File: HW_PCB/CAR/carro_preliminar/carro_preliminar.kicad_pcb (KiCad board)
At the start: 2 copper layers, 33 parts, among them IC1 TB6612FNG, J1 V_Battery, J2 STLINK, J3 Motores, J5 UART, J6 Servo_Motor, J7 NRF24_Con, SW1 SW_DPST_x2, U1 STM32F103C8Tx, U2 AMS1117-3.3, U3 AMS1117-3.3, Y1 8MHz

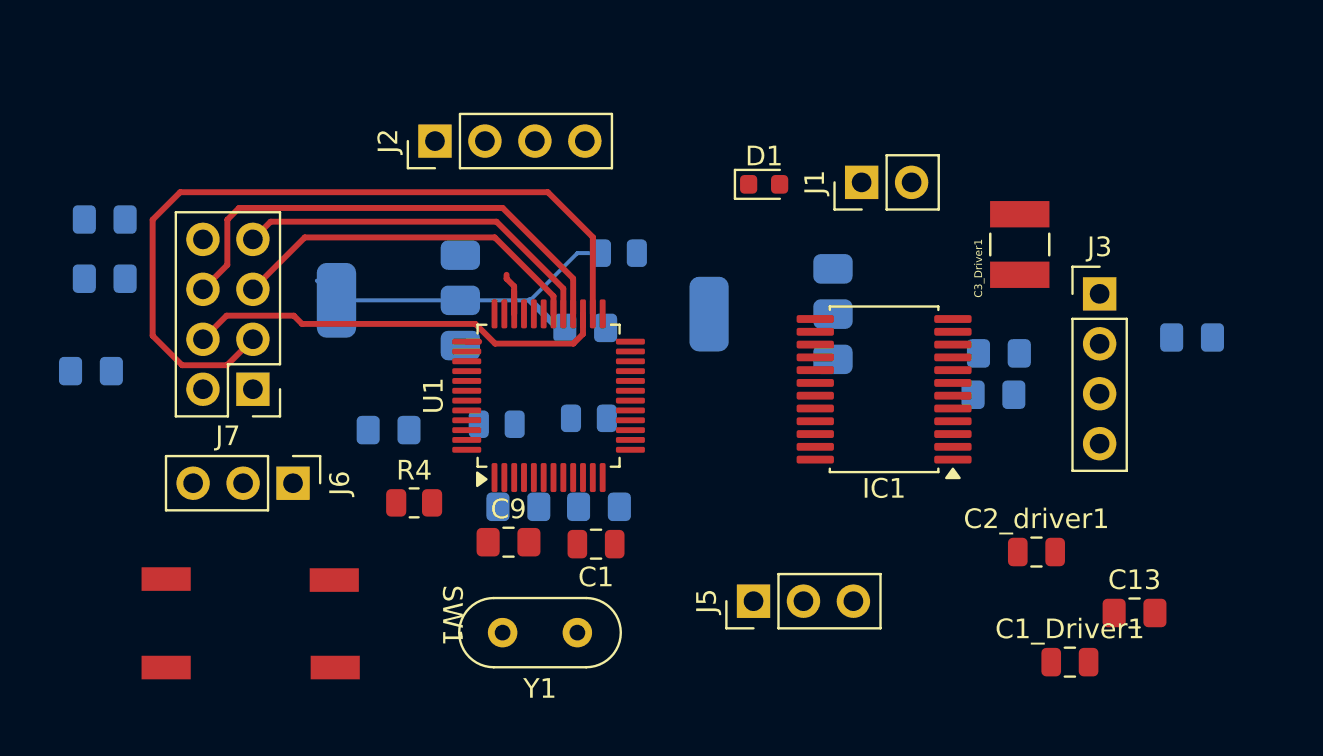
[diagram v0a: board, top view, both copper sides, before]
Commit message: Carrito 26-02-26
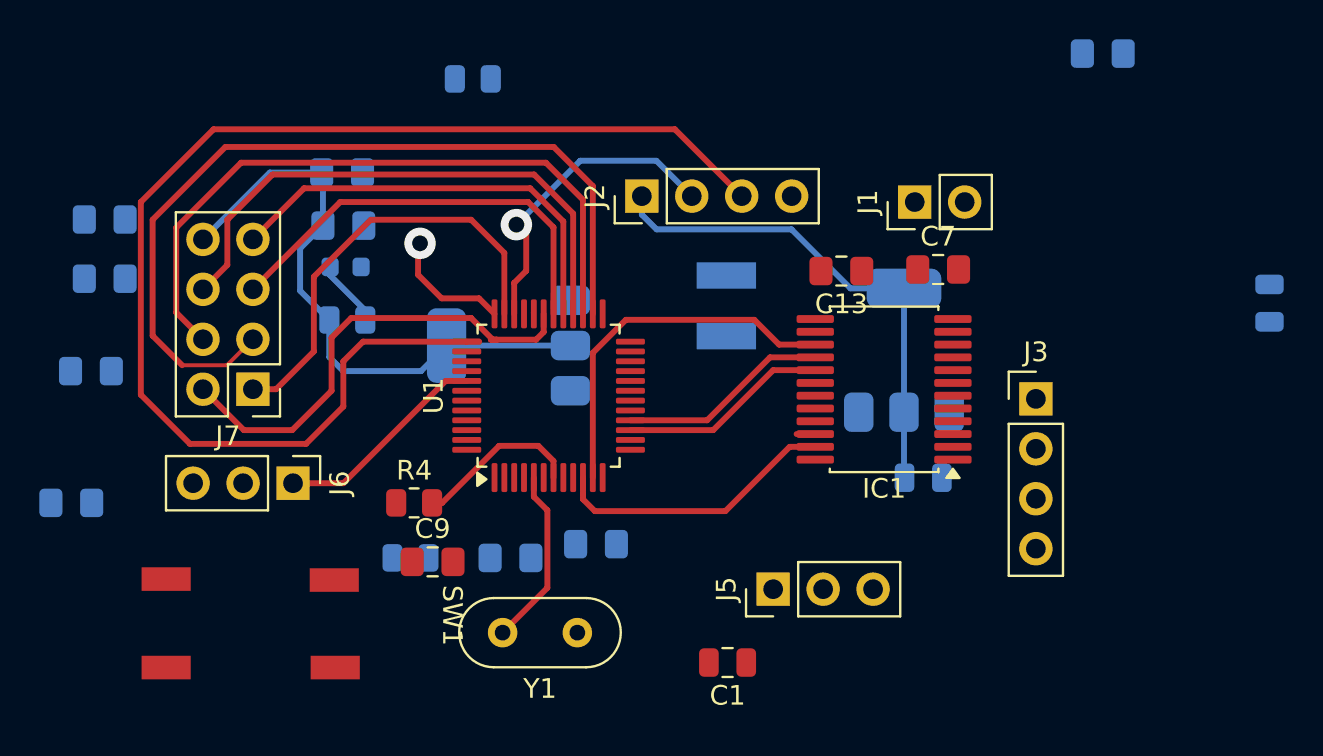
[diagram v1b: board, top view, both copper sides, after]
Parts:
- C1_Driver1, C2_driver1, C3_Driver1, D1: moved to B.Cu
- C7: moved to F.Cu
- moved C11 43.5 mm to (149.8, 78.0), turned to 0 degrees
- moved C13 22.9 mm to (175.1, 80.3), turned to 180 degrees
- moved D1 21.7 mm to (149.9, 80.1), turned to 180 degrees
- moved C1_Driver1 20.9 mm to (196.9, 81.9), turned to -90 degrees
- moved R1 18.2 mm to (156.4, 70.5)
- moved C8 16.6 mm to (136.0, 92.1)
- moved C12 16.1 mm to (188.4, 69.2)
- moved C3_Driver1 15.2 mm to (169.3, 82.1), turned to -90 degrees
- moved C10 14.7 mm to (149.7, 75.3)
- moved R3 14.2 mm to (150.0, 82.8)
- moved J2 10.9 mm to (165.0, 76.5)
- moved C1 9.00 mm to (169.3, 100.2)
- moved R2 8.09 mm to (153.2, 94.9)
- moved U2 7.01 mm to (178.3, 84.3), turned to 90 degrees
- moved C7 6.96 mm to (180.1, 80.2), turned to 0 degrees
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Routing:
- net SWCLK: track 0.63 -> 65.0 mm
- net VCC: track 0.00 -> 31.8 mm, vias 0 -> 1
- net PA10: track 0.00 -> 24.0 mm
- net GND: track 0.00 -> 22.4 mm
- net PA1: track 0.00 -> 18.9 mm
- net PA0: track 0.00 -> 14.5 mm
- net PB14: track 21.6 -> 34.9 mm
- net VCC_nrf24l01: track 18.2 -> 31.1 mm
- net SWDIO: track 3.32 -> 16.0 mm, vias 0 -> 1
- net PB5: track 0.00 -> 11.0 mm
- net PA6: track 0.00 -> 10.7 mm
- net PA5: track 0.00 -> 10.7 mm
- net OSC_IN: track 0.00 -> 9.12 mm
- net NRST: track 0.00 -> 8.54 mm
- net PA9: track 18.5 -> 22.1 mm
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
